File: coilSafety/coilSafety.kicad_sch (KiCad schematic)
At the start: 22 parts, among them J1 PJ-037BH, J10 Conn_01x02_Pin, J11 Conn_01x02_Pin, J2 Screw_Terminal_01x08, J3 Screw_Terminal_01x02, J4 Screw_Terminal_01x02, J5 Screw_Terminal_01x06, J6 Screw_Terminal_01x02, J7 Conn_01x01_Pin, J8 Conn_01x08_Pin, J9 Conn_01x02_Pin, K1 AZ943-1CH-12DE

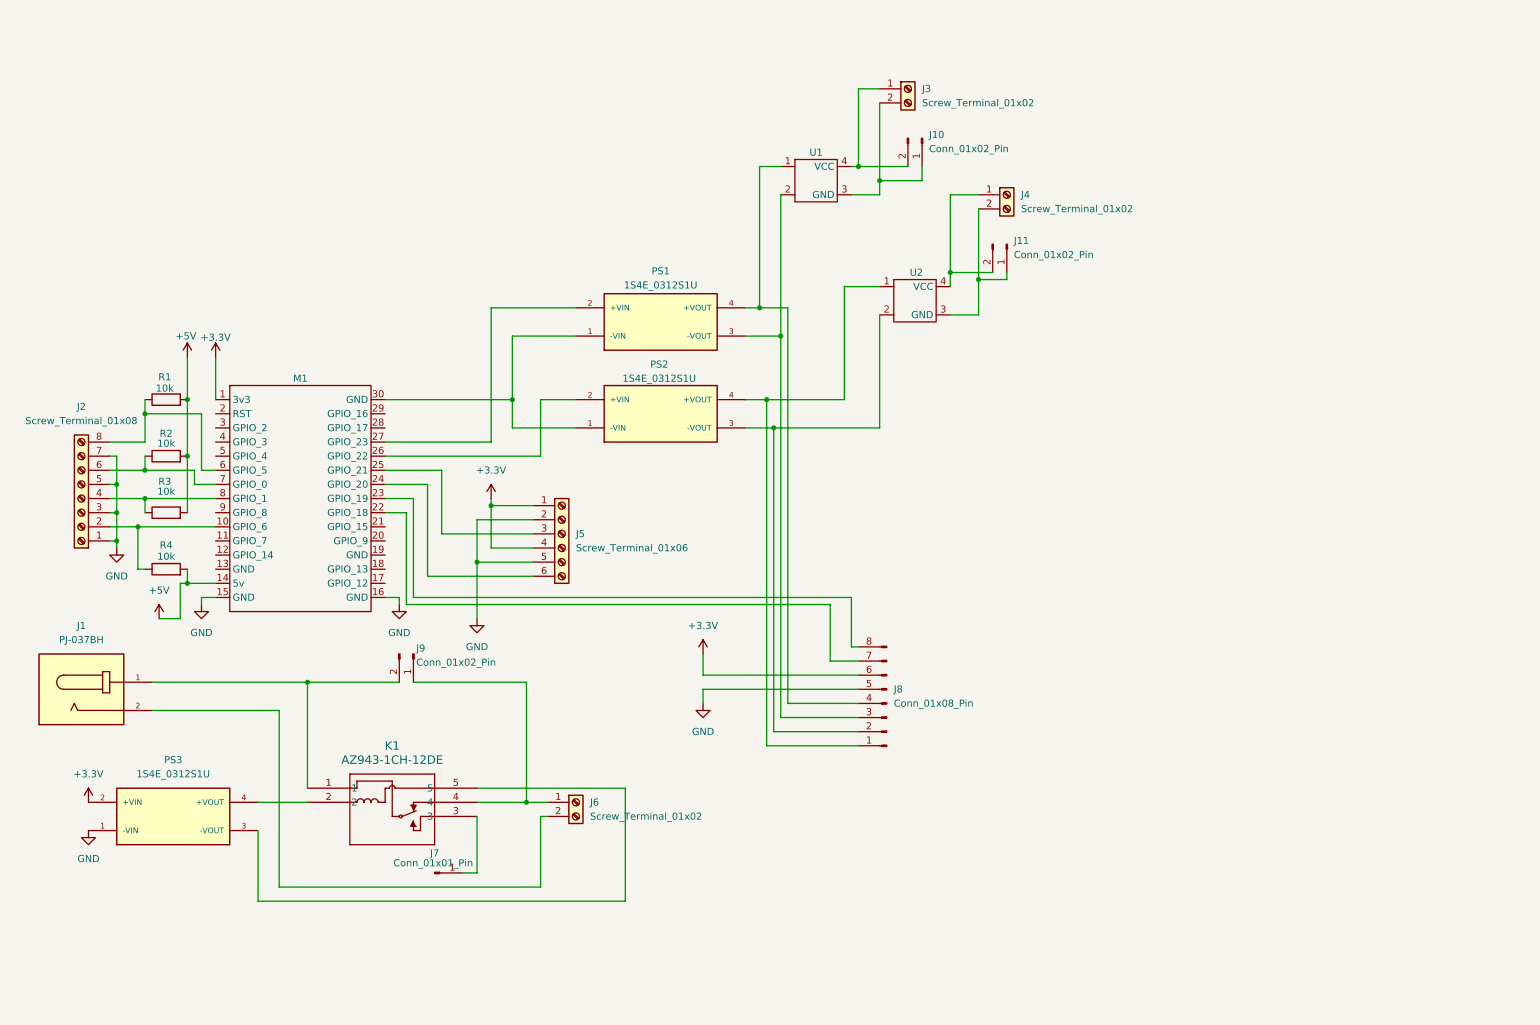
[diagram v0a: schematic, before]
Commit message: v2 schematic complete
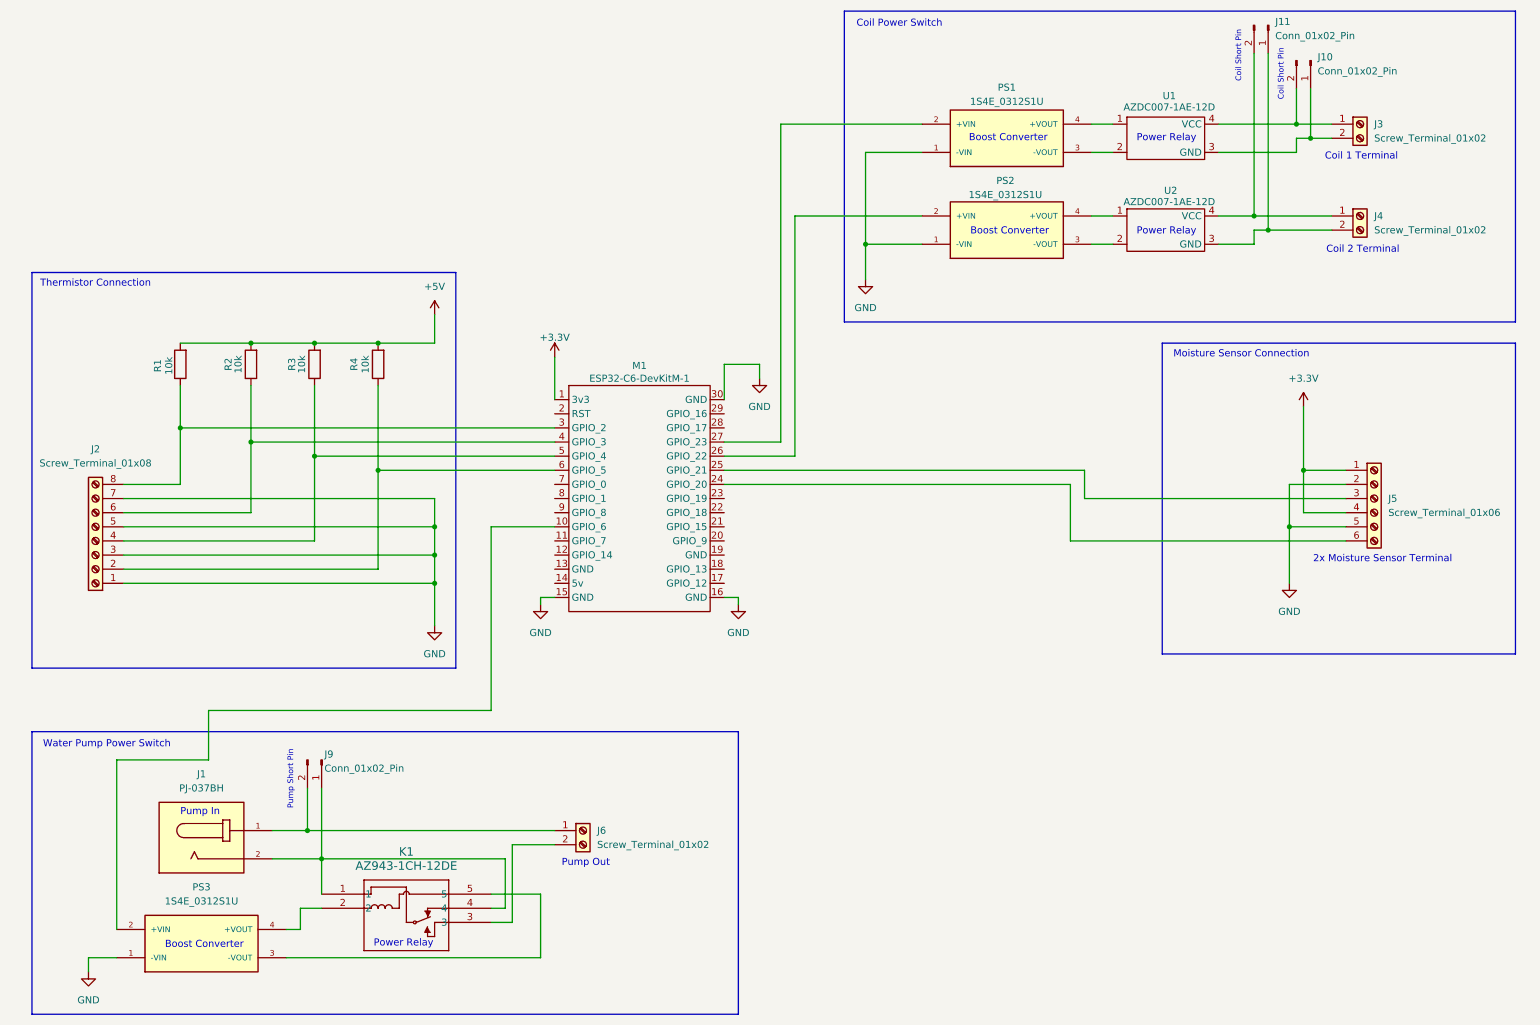
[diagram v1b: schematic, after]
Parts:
- removed J7: Conn_01x01_Pin, Connector_Samtec_HPM_THT:Samtec_HPM-01-01-x-S_Straight_1x01_Pitch5.08mm, symbol Connector:Conn_01x01_Pin
- removed J8: Conn_01x08_Pin, Connector_PinHeader_2.54mm:PinHeader_1x08_P2.54mm_Vertical, symbol Connector:Conn_01x08_Pin
- K1: footprint Footprints:AZ943-1CH-12DE -> AZ943-1CH_AMZ
- M1: value ~ -> ESP32-C6-DevKitM-1
- U1, U2: value ~ -> AZDC007-1AE-12D
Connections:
- net +3.3V: no longer PS3.2 (+VIN)
- net +5V: no longer M1.14 (5v)
- net GND: now also M1.30 (GND), PS1.1 (-VIN), PS2.1 (-VIN)
- net at J1.1, J9.2 (Pin_2): now also J6.1 (Pin_1); no longer K1.1
- net at J1.2: now also J9.1 (Pin_1), K1.1, K1.4; no longer J6.2 (Pin_2)
- net at J2.8 (Pin_8), R1.1: now also M1.3 (GPIO_2); no longer M1.6 (GPIO_5)
- net at J2.2 (Pin_2), R4.1: now also M1.6 (GPIO_5); no longer M1.10 (GPIO_6)
- net at J2.4 (Pin_4), R3.1: now also M1.5 (GPIO_4); no longer M1.8 (GPIO_1)
- net at J2.6 (Pin_6), R2.1: now also M1.4 (GPIO_3); no longer M1.7 (GPIO_0)
- net at K1.3: now also J6.2 (Pin_2)
- new net: M1.10 (GPIO_6), PS3.2 (+VIN)
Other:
- note added: "2x Moisture Sensor Terminal"
- note added: "Boost Converter"
- note added: "Coil 1 Terminal"
- note added: "Coil 2 Terminal"
- note added: "Coil Power Switch"
- note added: "Coil Short Pin"
- note added: "Moisture Sensor Connection"
- note added: "Power Relay"
- note added: "Pump In"
- note added: "Pump Out"
- note added: "Pump Short Pin"
- note added: "Thermistor Connection"
- note added: "Water Pump Power Switch"
- company: (none) -> Biedermann Lab
- title: (none) -> Coil Safety Circuit
- moved on the sheet: J1, J10, J11, J2, J3, J4, J5, J6, J9, K1, M1, PS1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
